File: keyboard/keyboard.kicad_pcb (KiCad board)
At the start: 2 copper layers, 98 x 143.5 mm, 79 parts, among them J5 Conn_01x15, J6 Conn_01x15, SW1 SW_Push, SW10 SW_Push, SW11 SW_Push, SW12 SW_Push, SW13 SW_Push, SW14 SW_Push, SW15 SW_Push, SW16 SW_Push, SW17 SW_Push, SW18 SW_Push, SW19 SW_Push, SW2 SW_Push, SW20 SW_Push, SW21 SW_Push, SW22 SW_Push, SW23 SW_Push, SW24 SW_Push, SW25 SW_Push, SW26 SW_Push, SW27 SW_Push, SW28 SW_Push, SW29 SW_Push, SW3 SW_Push, SW30 SW_Push, SW31 SW_Push, SW32 SW_Push, SW33 SW_Push, SW34 SW_Push, SW4 SW_Push, SW5 SW_Push, SW6 SW_Push, SW7 SW_Push, SW8 SW_Push, SW9 SW_Push

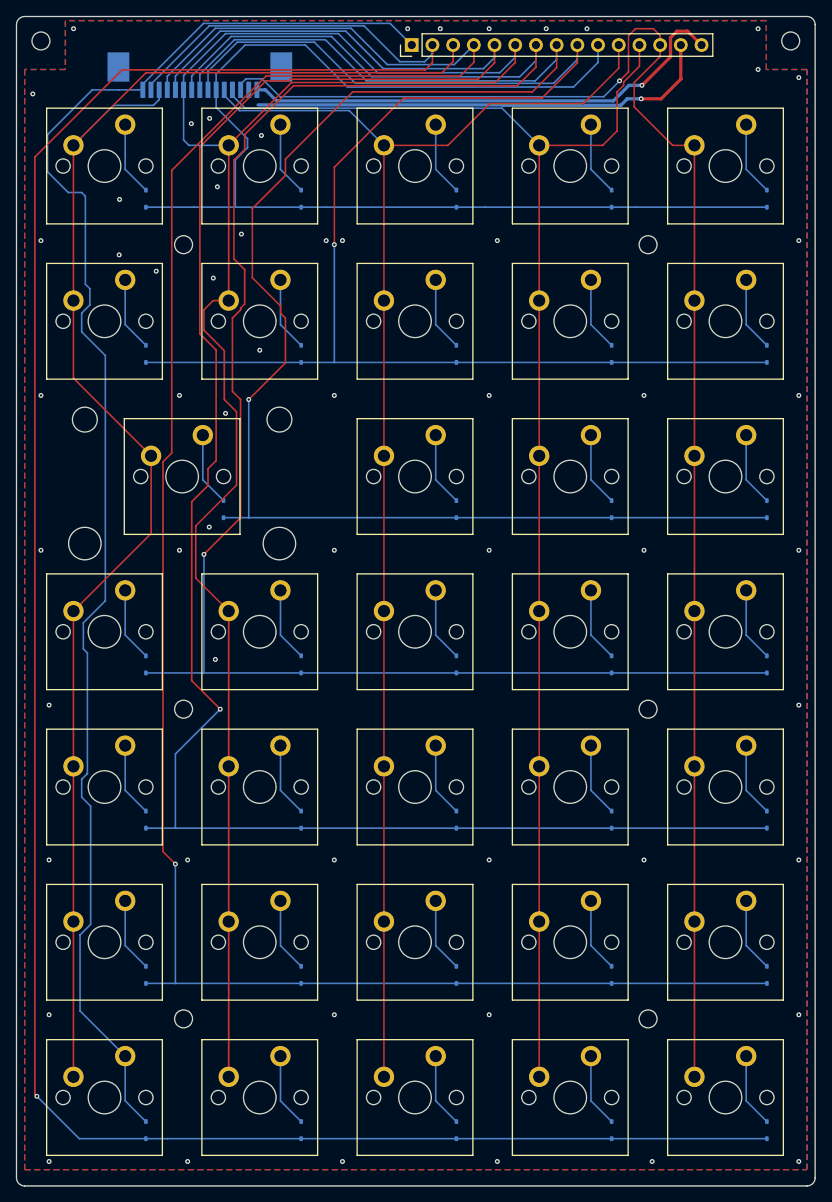
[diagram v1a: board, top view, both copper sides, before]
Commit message: all checks pass
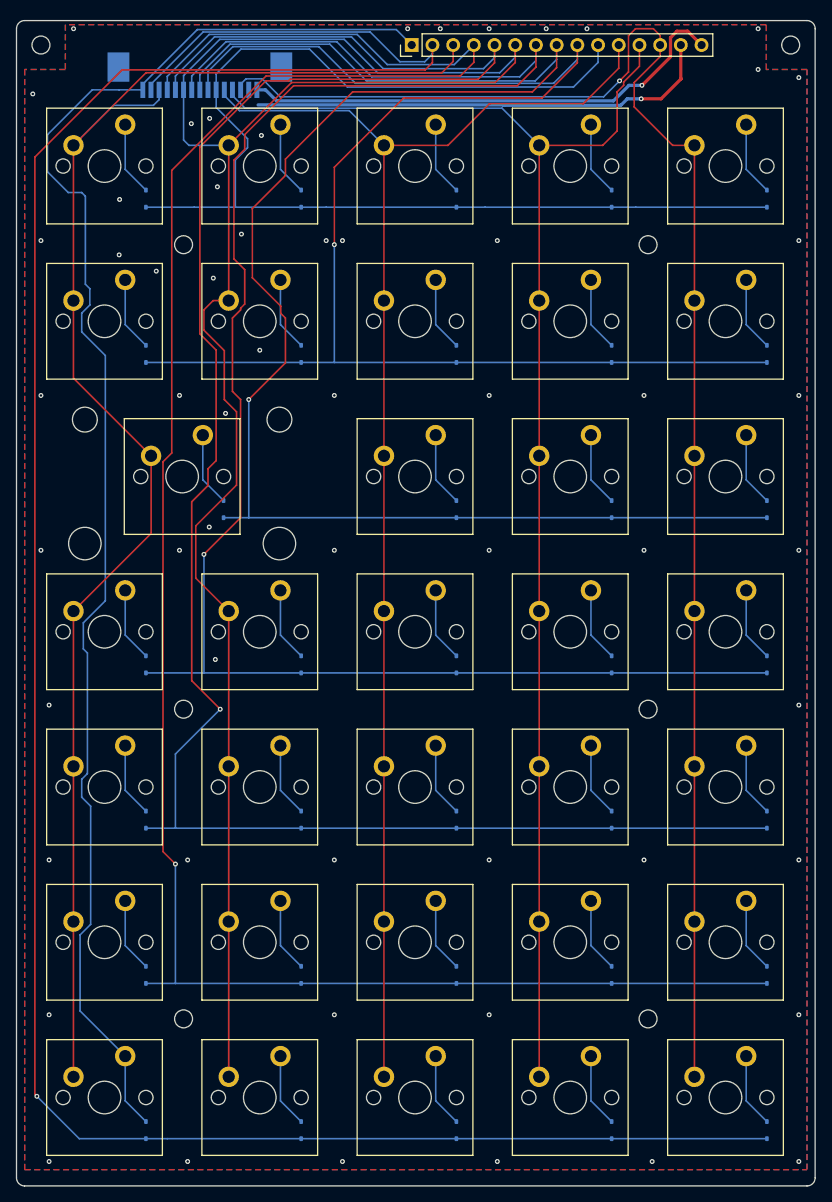
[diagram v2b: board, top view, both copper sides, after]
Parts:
- moved H3 0.50 mm to (154.0, 95.0)
- moved H4 0.50 mm to (62.0, 95.0)
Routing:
- net ROW5: track 266.3 -> 265.7 mm
- net WAKEUP: track 183.7 -> 183.0 mm
- net ROW6: track 304.4 -> 303.7 mm
- net ROW4: track 255.4 -> 254.8 mm
- net COL4: track 224.4 -> 223.8 mm
- net ROW3: track 238.9 -> 238.3 mm
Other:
- board size 98 x 143.5 mm -> 98 x 143 mm
